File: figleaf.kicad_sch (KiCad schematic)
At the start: 74 parts, among them J1 Conn_01x02_Pin, J2 HRO_TYPE-C-31-M-14, J3 Battery, J9 TC2030_SWD, Q2 2N7002, SW1 PWR, SW2 RST, U1 SRV05-4, U10 MAX17048, U3 BQ24075, U8 nRF52840_moko_mk08

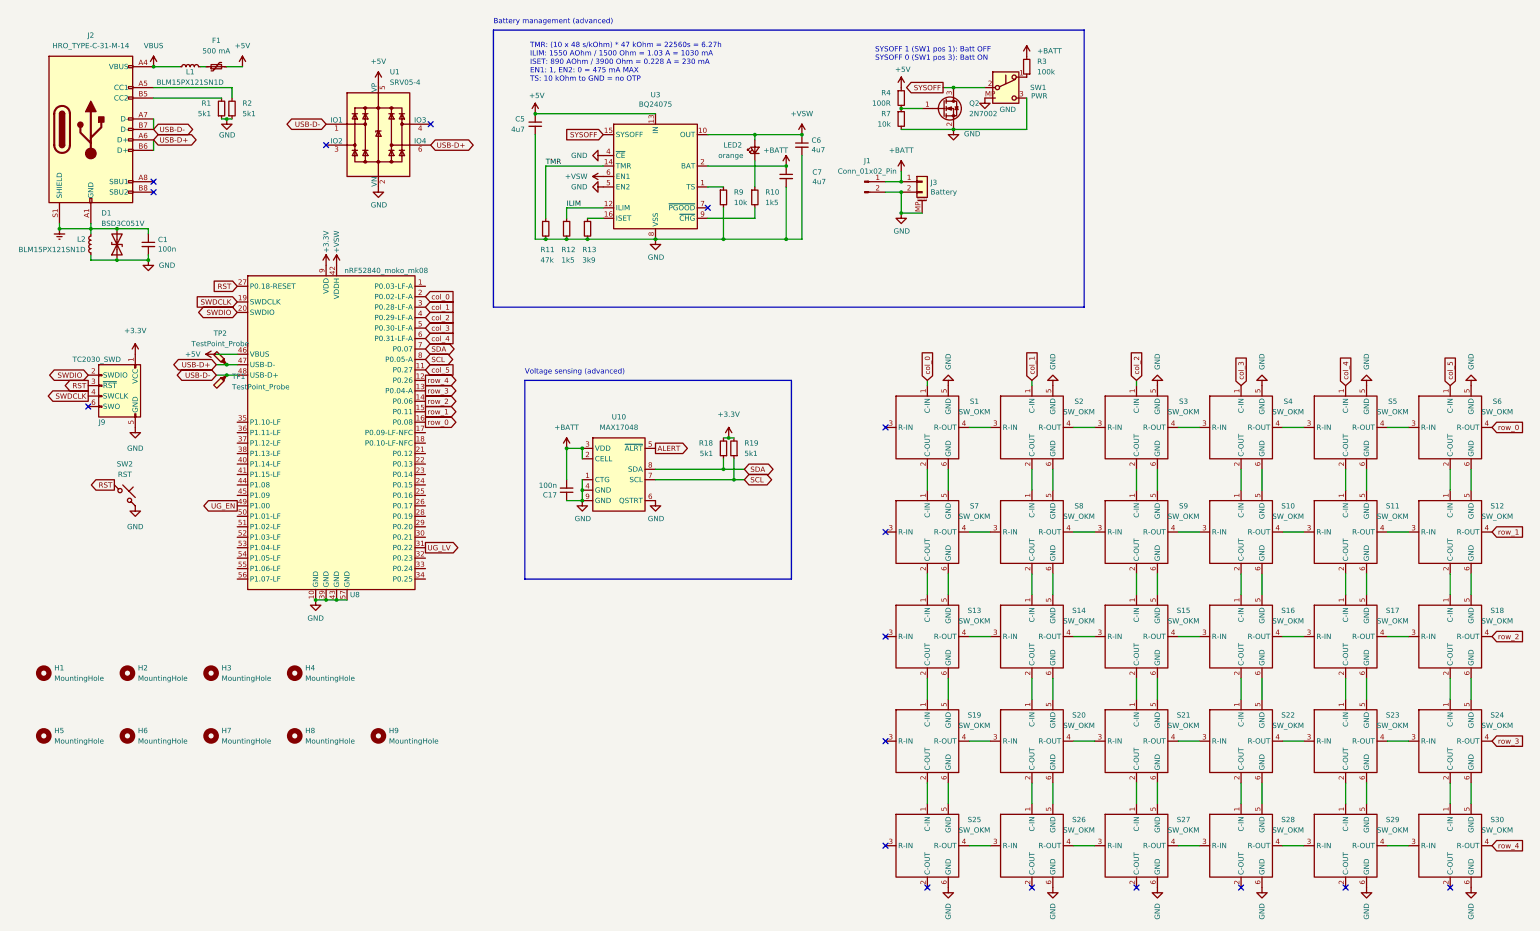
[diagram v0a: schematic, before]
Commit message: v1 progress
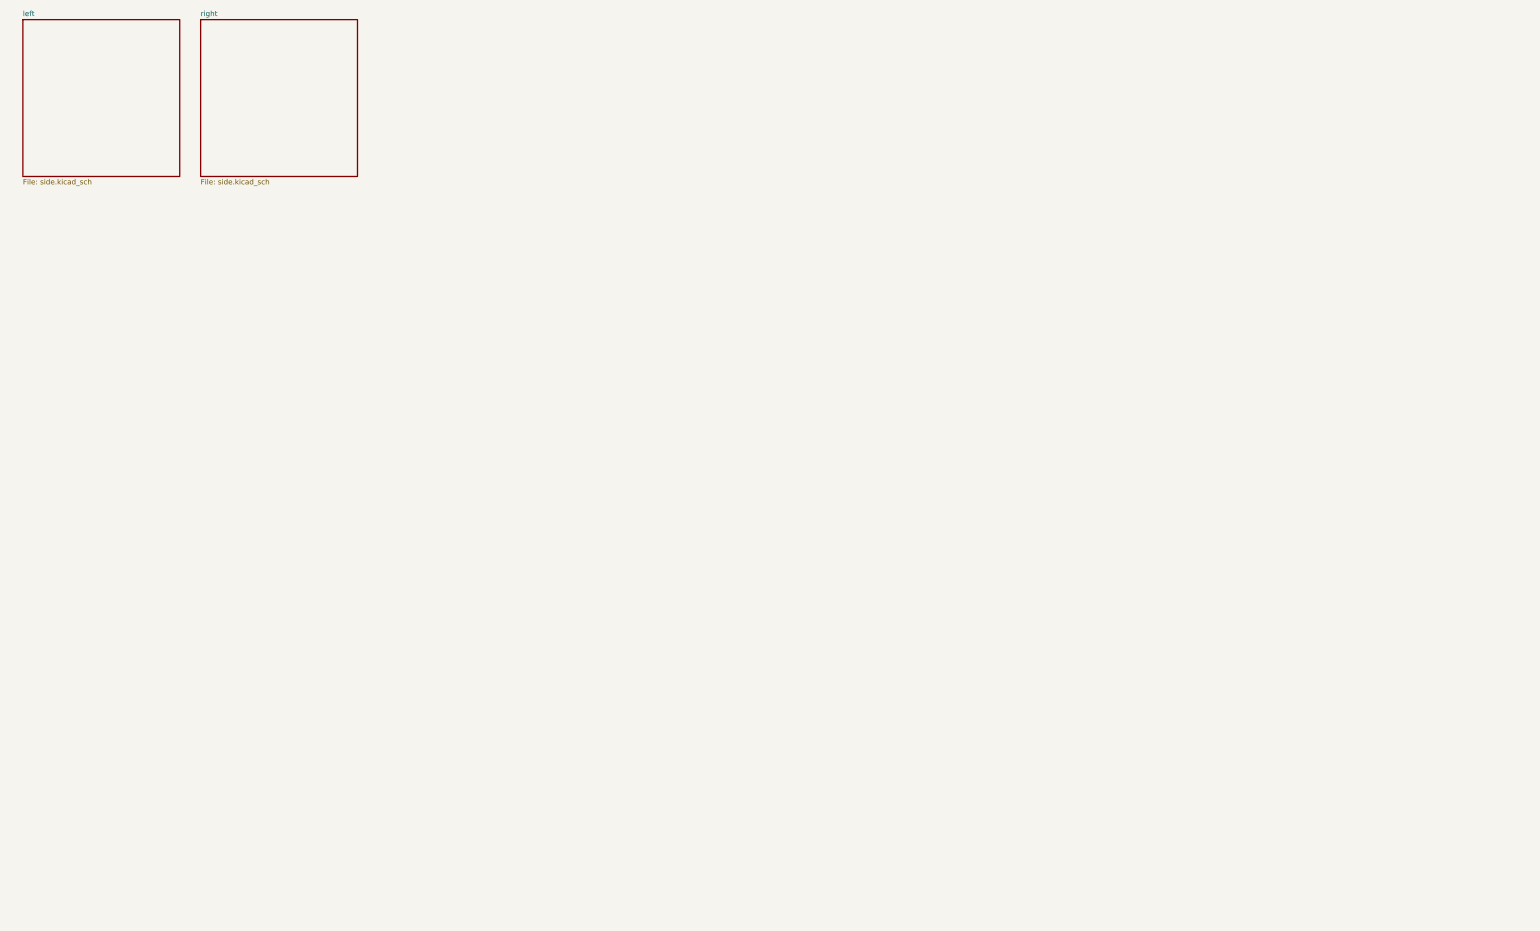
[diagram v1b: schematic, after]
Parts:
- removed C1, C17: 100n, Capacitor_SMD:C_0402_1005Metric, symbol Device:C_Small
- removed C5, C6, C7: 4u7, Capacitor_SMD:C_0402_1005Metric, symbol Device:C_Small
- removed D1: BSD3C051V, Diode_SMD:D_SOD-323, symbol Device:D_TVS
- removed F1: 500 mA, Fuse:Fuse_1206_3216Metric, symbol Device:Polyfuse_Small
- removed H1, H2, H3, H4, H5, H6, H7, H8, H9: MountingHole, Graz_Footprints:MountingHole_M2_Graz, symbol Mechanical:MountingHole
- removed J1: Conn_01x02_Pin, Graz_Footprints:Generic_Battery_Connector, symbol Connector:Conn_01x02_Pin
- removed J2: HRO_TYPE-C-31-M-14, PCM_marbastlib-various:USB_C_Receptacle_HRO_TYPE-C-31-M-14, symbol Connector:USB_C_Receptacle_USB2.0
- removed J3: Battery, Connector_JST:JST_SH_SM02B-SRSS-TB_1x02-1MP_P1.00mm_Horizontal, symbol Connector_Generic_MountingPin:Conn_01x02_MountingPin
- removed J9: TC2030_SWD, PCM_marbastlib-various:CON_TC2030_outlined, symbol PCM_marbastlib-various:TC2030_SWD
- removed L1, L2: BLM15PX121SN1D, Inductor_SMD:L_0402_1005Metric, symbol Device:L_Small
- removed LED2: orange, LED_SMD:LED_0402_1005Metric, symbol Device:LED_Small
- removed Q2: 2N7002, Package_TO_SOT_SMD:SOT-23, symbol Transistor_FET:2N7002
- removed R1, R18, R19, R2: 5k1, Resistor_SMD:R_0402_1005Metric, symbol Device:R_Small
- removed R10, R12: 1k5, Resistor_SMD:R_0402_1005Metric, symbol Device:R_Small
- removed R11: 47k, Resistor_SMD:R_0402_1005Metric, symbol Device:R_Small
- removed R13: 3k9, Resistor_SMD:R_0402_1005Metric, symbol Device:R_Small
- removed R3: 100k, Resistor_SMD:R_0402_1005Metric, symbol Device:R_Small
- removed R4: 100R, Resistor_SMD:R_0402_1005Metric, symbol Device:R_Small
- removed R7, R9: 10k, Resistor_SMD:R_0402_1005Metric, symbol Device:R_Small
- removed S1, S10, S11, S12, S13, S14, S15, S16, S17, S18, S19, S2, S20, S21, S22, S23, S24, S25, S26, S27, S28, S29, S3, S30, S4, S5, S6, S7, S8, S9: SW_OKM, Graz_Footprints:One Key Module Graz, symbol 0_graz_symbols:SW_OKM
- removed SW1: PWR, Graz_Footprints:SW_SSSS811101, symbol Switch:SW_Push_SPDT
- removed SW2: RST, Button_Switch_SMD:SW_SPST_B3U-3000P-B, symbol Switch:SW_Push_45deg
- removed TP1, TP2: TestPoint_Probe, TestPoint:TestPoint_Pad_D1.0mm, symbol Connector:TestPoint_Probe
- removed U1: SRV05-4, Package_TO_SOT_SMD:SOT-23-6, symbol Power_Protection:SRV05-4
- removed U10: MAX17048, Graz_Footprints:DFN-8-1EP_2x2mm_P0.5mm_EP0.7x1.3mm, symbol marbastlib-various:MAX17048
- removed U3: BQ24075, Package_DFN_QFN:VQFN-16-1EP_3x3mm_P0.5mm_EP1.6x1.6mm, symbol Battery_Management:BQ24075RGT
- removed U8: nRF52840_moko_mk08, Graz_Footprints:nRF52840_moko_mk08_GRAZ, symbol PCM_marbastlib-various:nRF52840_moko_mk08
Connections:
- no-connect marks 17 -> 0
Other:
- added sheet left (side.kicad_sch)
- added sheet right (side.kicad_sch)
- note removed: "Battery management (advanced)"
- note removed: "SYSOFF 1 (SW1 pos 1): Batt OFF SYSOFF 0 (SW1 pos 3): Batt ON"
- note removed: "TMR: (10 x 48 s/kOhm) * 47 kOhm = 22560s = 6.27h ILIM: 1550 AOhm / 1500 Ohm = 1.03 A = 1030 mA ISET: 890 AOhm / 3900 Ohm = 0.228 A = 230 mA EN1: 1, EN2: 0 = 475 mA MAX TS: 10 kOhm to GND = no OTP"
- note removed: "Voltage sensing (advanced)"
